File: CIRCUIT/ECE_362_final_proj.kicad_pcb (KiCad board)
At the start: 2 copper layers, 90.1 x 75.2 mm, 27 parts, among them J1 Conn_01x01_Pin, J2 Conn_01x01_Pin, J3 Conn_01x28_Socket, J4 Conn_01x28_Socket, SW2 BUTTON_MODE, SW4 BUTTON_CAPTURE, U1 TL084

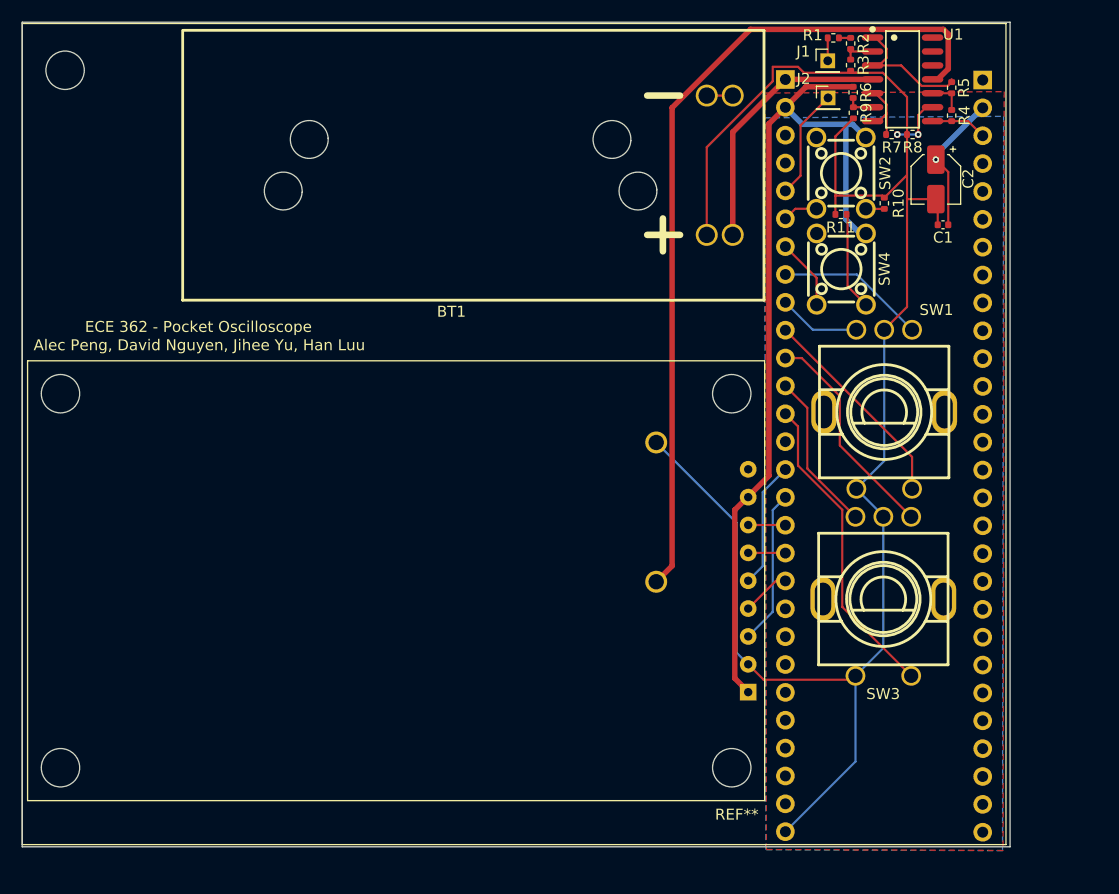
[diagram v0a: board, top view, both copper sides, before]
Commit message: PCB DONE
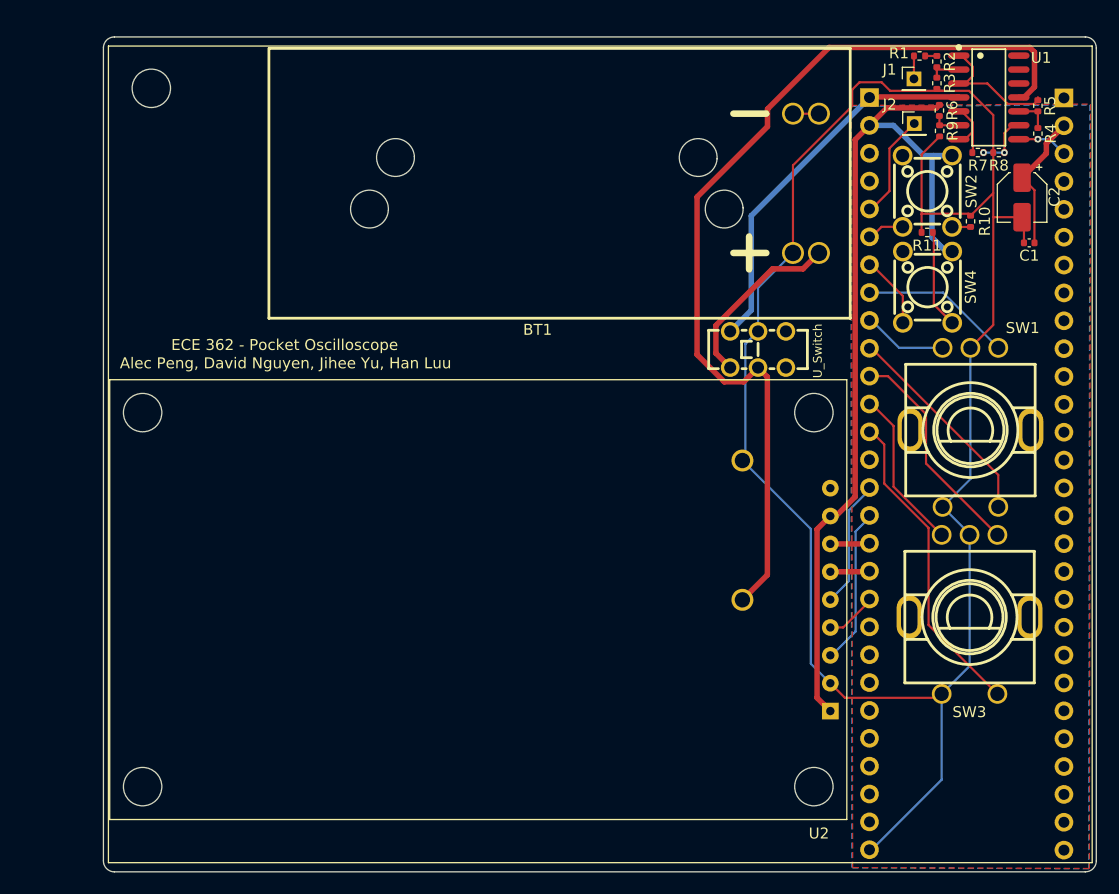
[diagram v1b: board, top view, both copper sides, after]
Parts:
- added U_Switch: SW-TH_SSSS222700, DPDT_switch:SW-TH_SSSS222700, F.Cu at (-0.23, 27.2)
- moved J2 8.20 mm to (14.0, 6.62)
- moved ? 8.03 mm to (-55.5, 3.41)
- moved BT2 8.03 mm to (2.96, 12.1)
- moved C2 8.03 mm to (23.8, 13.4)
- moved J1 8.03 mm to (14.0, 2.55)
- moved R1 8.03 mm to (14.5, 0.46)
- moved R10 8.03 mm to (19.1, 15.5)
- moved R2 8.03 mm to (16.1, 0.97)
- moved R3 8.03 mm to (16.1, 2.95)
- moved R4 8.03 mm to (25.3, 7.54)
- moved R5 8.03 mm to (25.3, 5.00)
- moved R6 8.03 mm to (16.3, 5.43)
- moved R9 8.03 mm to (16.3, 7.29)
- moved SW3 8.03 mm to (19.1, 51.4)
- moved SW4 8.03 mm to (15.2, 21.5)
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- gave numbers to parts that had none: 1
- renumbered REF** to U2
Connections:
- BT1 pad 2: +BATT -> BT1+
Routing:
- net GND: track 161.5 -> 183.3 mm
- net BT1+: track 0.00 -> 16.5 mm
- net +BATT: track 24.1 -> 34.8 mm
- net -BATT: track 77.1 -> 86.5 mm
- net /GPIO2: track 10.2 -> 9.48 mm
- net +3.3V: track 95.0 -> 94.5 mm, vias 1 -> 0
- net /GPIO47_ADC7: track 5.12 -> 4.66 mm, vias 0 -> 1
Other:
- board size 90.1 x 75.2 mm -> 90.5 x 76.1 mm
